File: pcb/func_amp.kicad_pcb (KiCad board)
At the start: 2 copper layers, 86 x 50 mm, 41 parts, among them J1 PWR, J2 IN, J3 LOAD, P1 AC-01B, T1 ST-6-20, U1 L7815, U2 L7915, U3 TDA2030

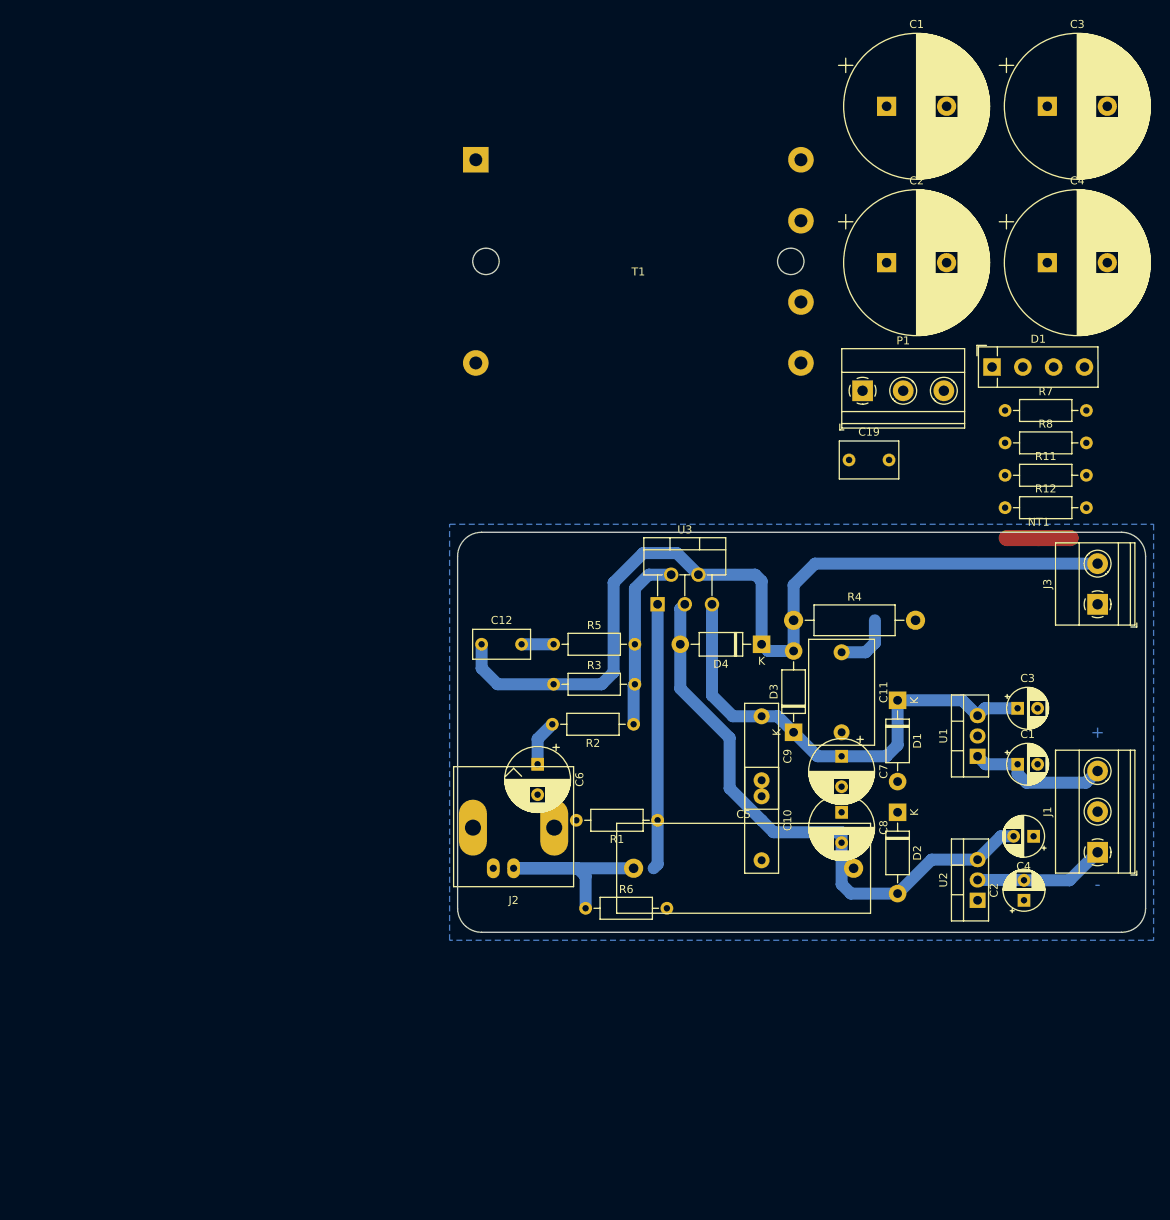
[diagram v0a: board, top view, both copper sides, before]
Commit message: pcb layout
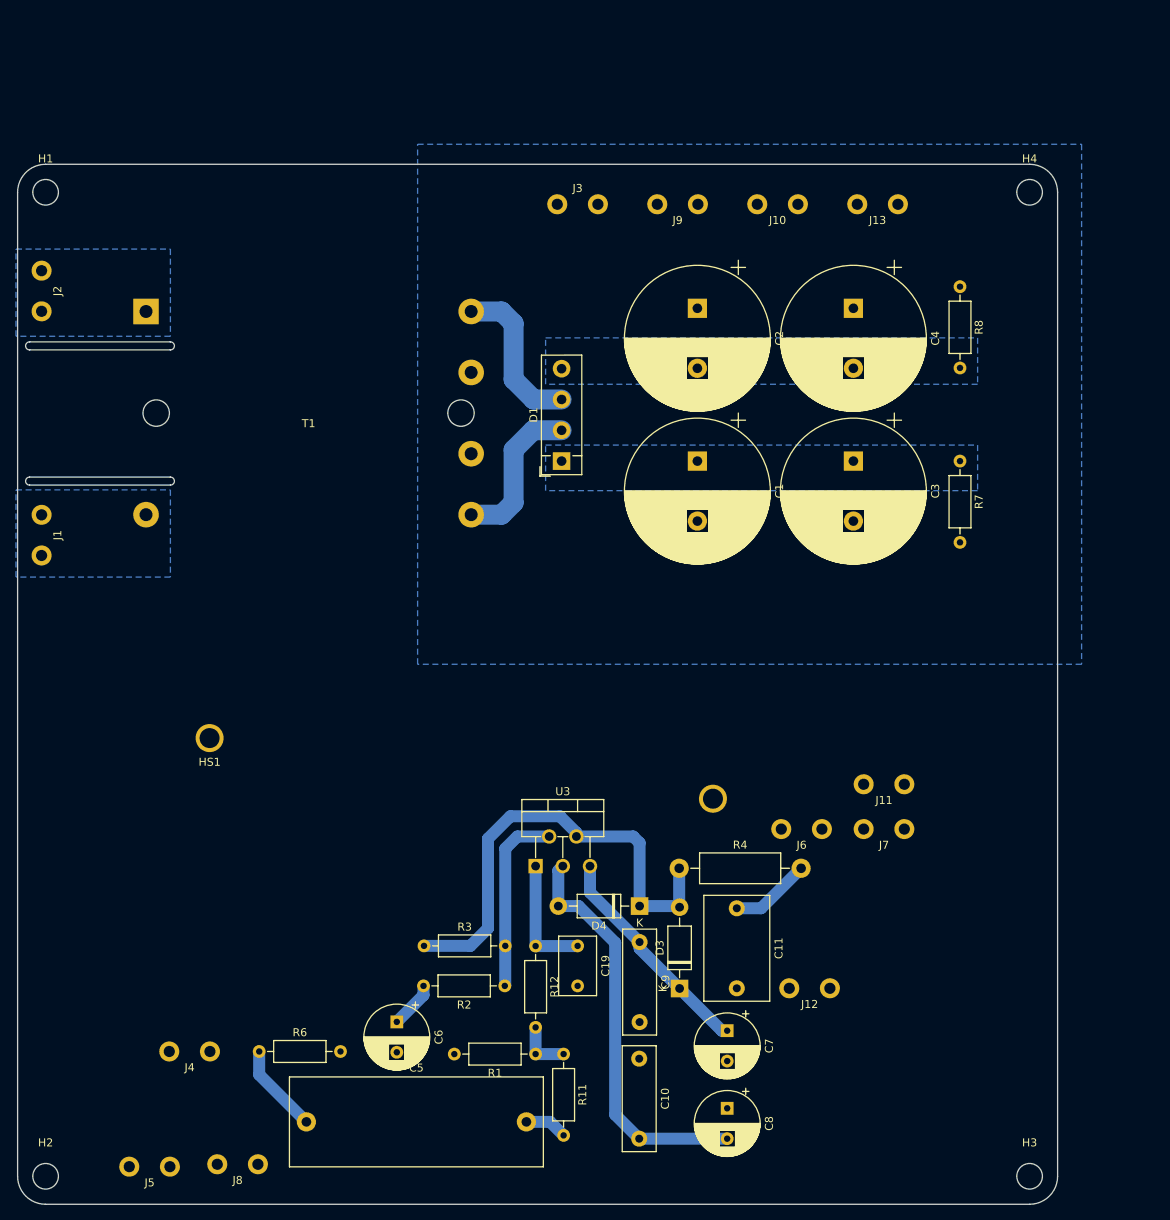
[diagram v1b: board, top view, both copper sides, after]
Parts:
- removed the C1 at (158.6, 17.8)
- removed the C1 at (175.0, 100.0)
- removed C12: 2.2n, Capacitor_THT:C_Rect_L7.0mm_W3.5mm_P5.00mm
- removed the C2 at (158.6, 37.3)
- removed the C2 at (175.8, 117.0)
- removed the C3 at (178.7, 17.8)
- removed the C3 at (175.0, 93.0)
- removed the C4 at (178.7, 37.3)
- removed the C4 at (177.0, 109.0)
- removed the D1 at (171.8, 50.3)
- removed the D1 at (160.0, 92.0)
- removed D2: 1N4001, Diode_THT:D_DO-41_SOD81_P10.16mm_Horizontal
- removed NT1: Net-Tie_3_Tee, NetTie:NetTie-3_SMD_Pad2.0mm
- removed P1: AC-01B, TerminalBlock_Phoenix:TerminalBlock_Phoenix_MKDS-1,5-3-5.08_1x03_P5.08mm_Horizontal
- removed R5: 3R2, Resistor_THT:R_Axial_DIN0207_L6.3mm_D2.5mm_P10.16mm_Horizontal
- removed U1: L7815, Package_TO_SOT_THT:TO-220-3_Vertical
- removed U2: L7915, Package_TO_SOT_THT:TO-220-3_Vertical
- added C1: 3300uF, Capacitor_THT:CP_Radial_D18.0mm_P7.50mm, F.Cu at (135.0, 62.1)
- added C2: 3300uF, Capacitor_THT:CP_Radial_D18.0mm_P7.50mm, F.Cu at (135.0, 43.0)
- added C3: 3300uF, Capacitor_THT:CP_Radial_D18.0mm_P7.50mm, F.Cu at (154.5, 62.1)
- added C4: 3300uF, Capacitor_THT:CP_Radial_D18.0mm_P7.50mm, F.Cu at (154.5, 43.0)
- added D1: KBP10G, Diode_THT:Diode_Bridge_Vishay_KBPM, F.Cu at (118.0, 62.1)
- added H1: MountingHole, MountingHole:MountingHole_3.2mm_M3, F.Cu at (53.5, 28.5)
- added H2: MountingHole, MountingHole:MountingHole_3.2mm_M3, F.Cu at (53.5, 151.5)
- added H3: MountingHole, MountingHole:MountingHole_3.2mm_M3, F.Cu at (176.5, 151.5)
- added H4: MountingHole, MountingHole:MountingHole_3.2mm_M3, F.Cu at (176.5, 28.5)
- added HS1: Heatsink, pl_heatsink:random_psu_heatsink, F.Cu at (74.0, 96.7)
- added J10: GNDS, pl_connector:TE_0.25in_spade_63824-1, F.Cu at (145.0, 30.0)
- added J11: GND, pl_connector:TE_0.25in_spade_63824-1, F.Cu at (158.3, 102.5)
- added J12: GNDPWR, pl_connector:TE_0.25in_spade_63824-1, F.Cu at (149.0, 128.0)
- added J13: GNDPWR, pl_connector:TE_0.25in_spade_63824-1, F.Cu at (157.5, 30.0)
- added J4: IN, pl_connector:TE_0.25in_spade_63824-1, F.Cu at (71.5, 135.9)
- added J5: GNDS, pl_connector:TE_0.25in_spade_63824-1, F.Cu at (66.5, 150.3)
- added J6: OUT, pl_connector:TE_0.25in_spade_63824-1, F.Cu at (148.0, 108.1)
- added J7: GND, pl_connector:TE_0.25in_spade_63824-1, F.Cu at (158.3, 108.1)
- added J8: GNDS, pl_connector:TE_0.25in_spade_63824-1, F.Cu at (77.5, 150.0)
- added J9: GND, pl_connector:TE_0.25in_spade_63824-1, F.Cu at (132.5, 30.0)
- J1: value PWR -> L; footprint TerminalBlock_Phoenix:TerminalBlock_Phoenix_MKDS-1,5-3-5.08_1x03_P5.08mm_Horizontal -> pl_connector:TE_0.25in_spade_63824-1
- J2: value IN -> N; footprint Connector_Coaxial:BNC_Amphenol_B6252HB-NPP3G-50_Horizontal -> pl_connector:TE_0.25in_spade_63824-1
- J3: value LOAD -> G; footprint TerminalBlock_Phoenix:TerminalBlock_Phoenix_MKDS-1,5-2-5.08_1x02_P5.08mm_Horizontal -> pl_connector:TE_0.25in_spade_63824-1
- moved J1 137.8 mm to (53.0, 71.4)
- moved J2 93.2 mm to (53.0, 40.8), turned to 90 degrees
- moved R11 91.0 mm to (118.2, 136.2), turned to 270 degrees
- moved J3 82.0 mm to (120.0, 30.0), turned to 180 degrees
- moved R12 80.3 mm to (114.8, 122.7), turned to 270 degrees
- moved C19 69.6 mm to (120.0, 122.7), turned to 270 degrees
- moved C5 51.7 mm to (86.1, 144.7)
- moved T1 45.4 mm to (86.4, 56.1)
- moved R6 44.6 mm to (80.2, 135.9)
- moved C8 39.7 mm to (138.7, 143.0)
- moved C10 38.0 mm to (127.7, 136.8)
- moved C7 37.2 mm to (138.7, 133.3)
- moved C6 36.7 mm to (97.4, 132.2)
- moved R3 36.5 mm to (100.8, 122.7)
- moved R2 36.4 mm to (110.9, 127.7)
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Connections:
- J1 pad 1: /-V -> /L
- J2 pad 1: Net-(C5-Pad1) -> /N
- J3 pad 1: GND -> Earth
- R7 pad 2: GNDPWR -> Earth
- R8 pad 1: GNDPWR -> Earth
- T1 pad 6: GNDPWR -> Earth
- T1 pad 7: GNDPWR -> Earth
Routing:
- net Net-(C12-Pad1): track 113.2 -> 0.00 mm
- net -15V: track 73.5 -> 0.00 mm
- net +15V: track 60.1 -> 0.00 mm
- net Net-(D3-Pad2): track 0.00 -> 59.7 mm
- net -V: track 0.00 -> 51.0 mm
- net Net-(C5-Pad1): track 42.0 -> 11.2 mm
- net +V: track 0.00 -> 28.1 mm
- net Net-(C5-Pad2): track 33.2 -> 5.35 mm
- net Net-(D1-Pad3): track 0.00 -> 20.0 mm
- net Net-(D1-Pad2): track 0.00 -> 19.5 mm
- net /+V: track 17.7 -> 0.00 mm
- net /-V: track 16.5 -> 0.00 mm
- net Net-(C19-Pad1): track 0.00 -> 15.3 mm
- net Net-(R1-Pad1): track 0.00 -> 6.84 mm
- net Net-(C12-Pad2): track 4.00 -> 0.00 mm
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- added copper zone on B.Cu, net +V
- added copper zone on B.Cu, net -V
- added copper zone on B.Cu, net /L
- added copper zone on B.Cu, net /N
- added copper zone on B.Cu, net Earth
- removed copper zone on B.Cu, net GND
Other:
- board size 86 x 50 mm -> 130 x 130 mm
- board text removed: "+"
- board text removed: "-"
